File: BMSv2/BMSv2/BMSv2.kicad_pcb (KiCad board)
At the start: 2 copper layers, 44.6 x 41.2 mm, 126 parts, among them J1 Conn_01x05, J2 Conn_01x04_Socket, J3 Conn_01x02_Pin, J4 Conn_01x02_Pin, J5 Conn_01x03_Pin, Q1 AO3401A, Q10 MMBT3904, Q11 MMBT3904, Q12 MMBT3904, Q13 MMBT3904, Q14 Q_PNP_BEC, Q15 Q_PNP_BEC, Q16 Q_PNP_BEC, Q17 Q_PNP_BEC, Q2 MMBT3904, Q3 DMG2301L, Q4 MMBT3904, Q5 DMG2301L, Q6 MMBT3904, Q7 DMG2301L, Q8 MMBT3904, Q9 DMG2301L, SW1 SW_BOOT0, U1 STM32F405RGTx, U2 MCP2561-E-SN, U4 MP2332H, U5 AMS1117-3.3, Y1 Crystal_16MHz

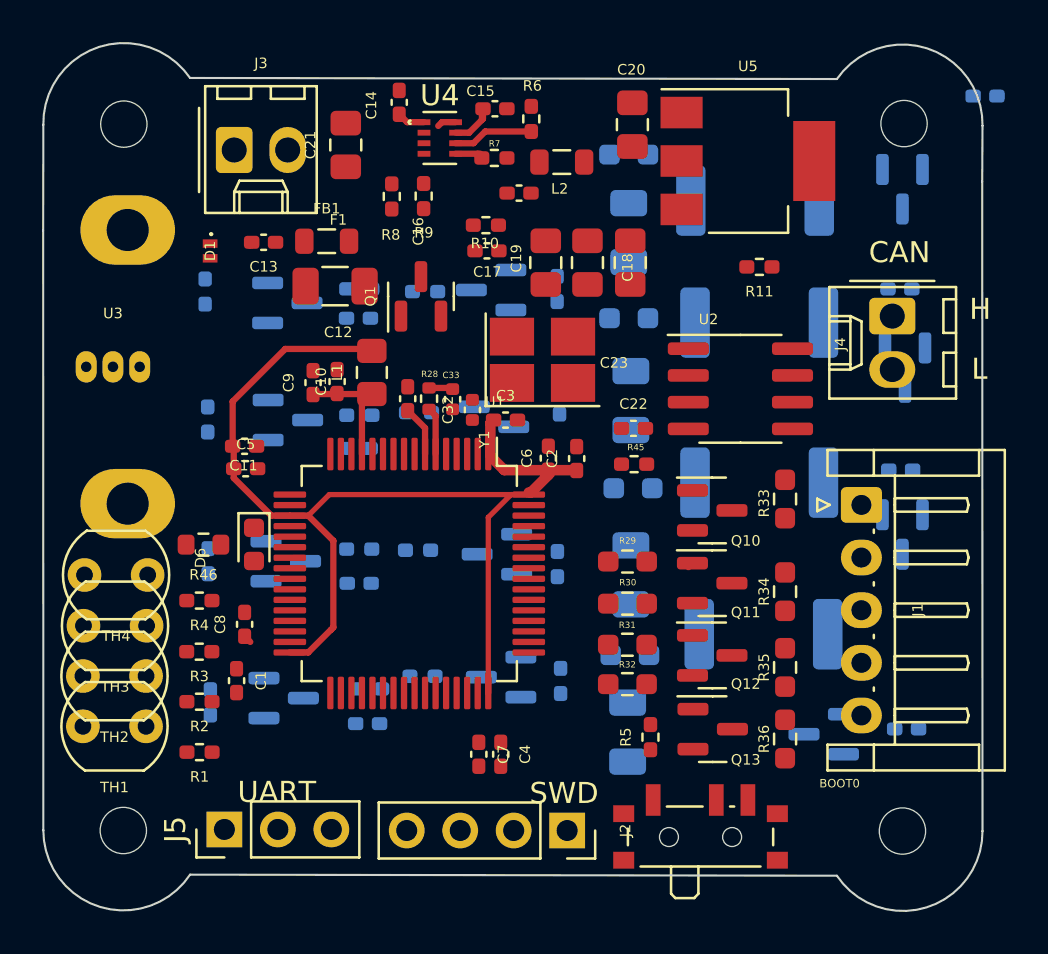
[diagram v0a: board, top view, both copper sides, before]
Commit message: Add files via upload
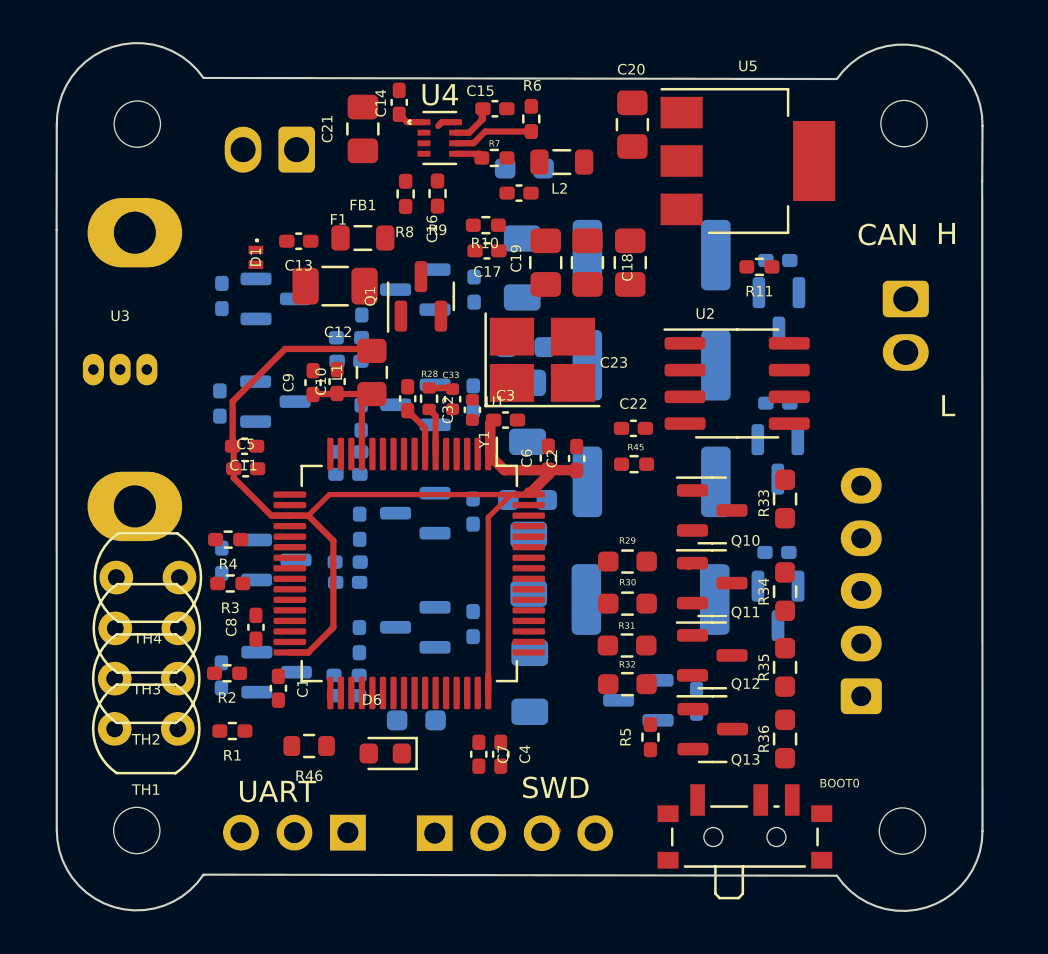
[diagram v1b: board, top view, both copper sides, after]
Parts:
- J1, J2, J3, J4, J5: moved to B.Cu
- moved C24 12.6 mm to (103.7, 53.8)
- moved D6 11.7 mm to (85.0, 77.3), turned to 180 degrees
- moved R46 10.8 mm to (81.4, 76.9)
- moved R40 10.6 mm to (86.5, 75.7), turned to 180 degrees
- moved C27 10.1 mm to (99.8, 74.8), turned to 90 degrees
- moved J1 9.09 mm to (107.6, 74.5), turned to 90 degrees
- moved Q17 8.95 mm to (97.1, 74.7)
- moved Q14 8.29 mm to (103.7, 56.3)
- moved C25 7.94 mm to (103.7, 60.6)
- moved Q15 7.45 mm to (103.7, 63.3)
- moved C26 7.06 mm to (103.6, 67.7)
- moved Q16 6.81 mm to (103.7, 70.3)
- moved J2 6.29 mm to (87.4, 81.1)
- moved J5 5.87 mm to (83.3, 81.0)
- moved R44 5.61 mm to (97.6, 70.0)
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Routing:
- net SWDIO: track 0.59 -> 0.00 mm
- net +3.3V: track 54.0 -> 54.6 mm
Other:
- board size 44.6 x 41.2 mm -> 44 x 41.2 mm
